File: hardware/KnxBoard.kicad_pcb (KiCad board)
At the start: 4 copper layers, 41.8 x 41.9 mm, 47 parts, among them IC0 STM32G491KEU6, IC1 NCN5130, J1 Conn_01x16, J2 Conn_01x16, J4 Conn_01x02_Male, X1 FA-238

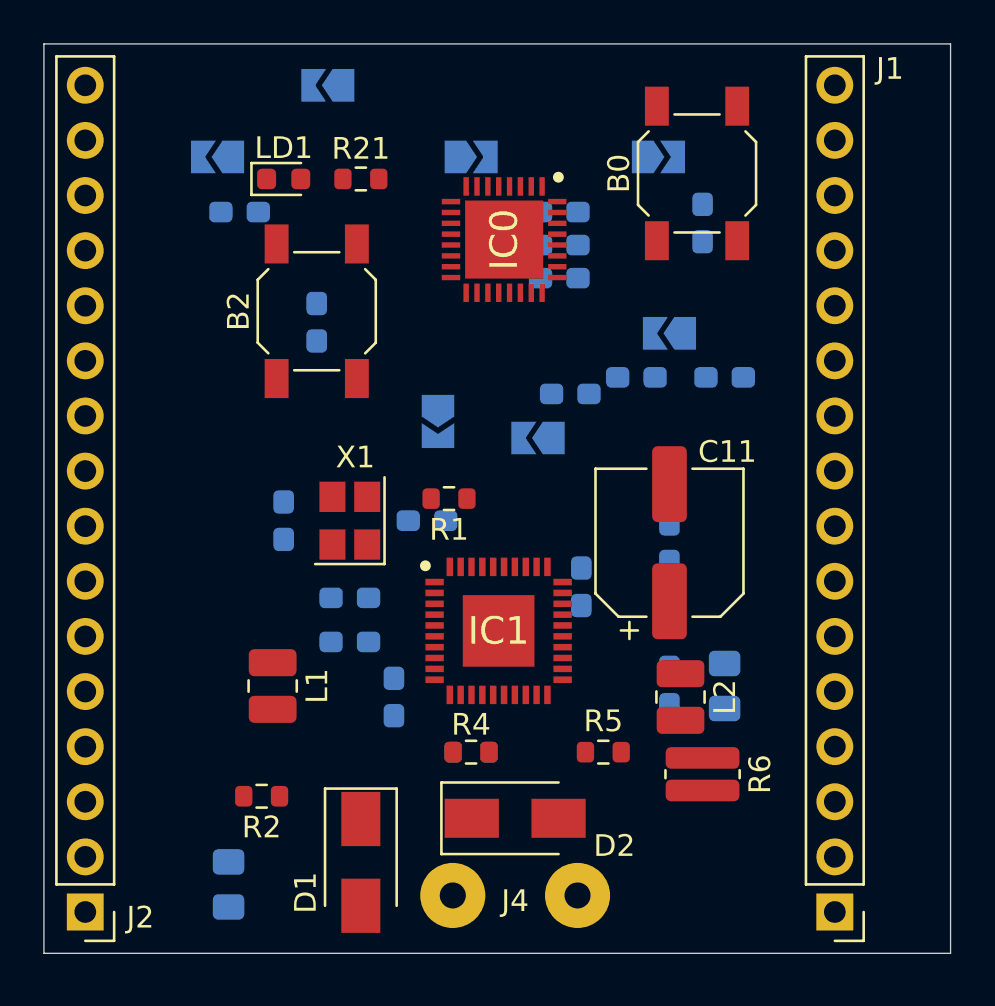
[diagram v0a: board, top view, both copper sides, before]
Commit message: Routage OK need check and mass and texts
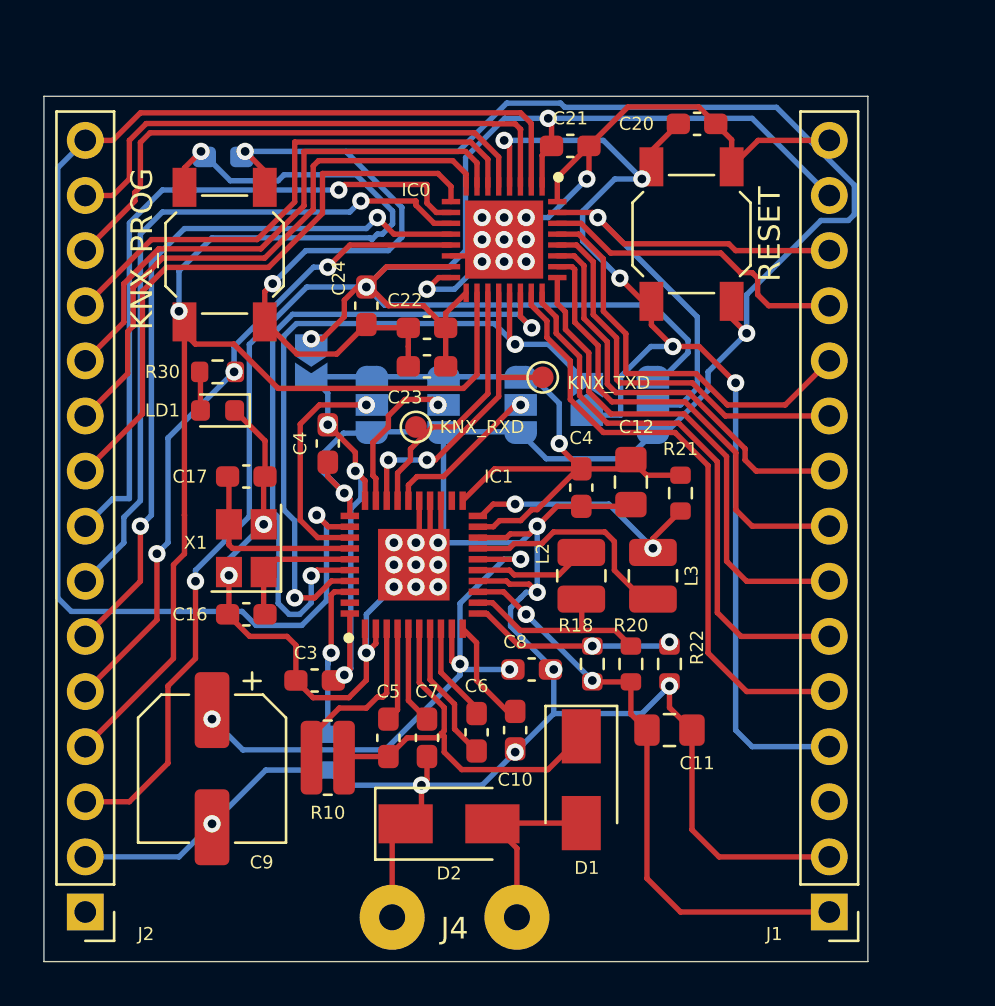
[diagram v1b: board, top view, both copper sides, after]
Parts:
- removed C1 (x2): 100 nF, Capacitor_SMD:C_0603_1608Metric_Pad1.08x0.95mm_HandSolder
- removed the C11 at (113.3, 55.4)
- removed C5_9: 100nF, Capacitor_SMD:C_0603_1608Metric_Pad1.08x0.95mm_HandSolder
- removed JP0, JP5: Bootloader, Jumper:SolderJumper-2_P1.3mm_Open_TrianglePad1.0x1.5mm
- added C20: 100 nF, Capacitor_SMD:C_0603_1608Metric_Pad1.08x0.95mm_HandSolder, F.Cu at (114.6, 36.1)
- added C8: 100nF 50V, Capacitor_SMD:C_0603_1608Metric_Pad1.08x0.95mm_HandSolder, F.Cu at (106.9, 61.2)
- added C9: 100uF 35V, Capacitor_SMD:CP_Elec_6.3x7.7, F.Cu at (92.2, 65.8)
- added JP3: Speed, Jumper:SolderJumper-3_P1.3mm_Open_RoundedPad1.0x1.5mm, B.Cu at (106.4, 49.0)
- added TP1: KNX_RXD, TestPoint:TestPoint_Pad_D1.0mm, F.Cu at (101.6, 50.0)
- added TP2: KNX_TXD, TestPoint:TestPoint_Pad_D1.0mm, F.Cu at (107.4, 47.8)
- C10: renamed from C12; value 1uF 35V ESR < 2ohm -> 1uF 50V ESR < 2ohm; moved to F.Cu
- C11: renamed from C19; moved to F.Cu
- C12: renamed from C20; moved to F.Cu
- C16, C17, C4: moved to F.Cu
- C21: renamed from C5; moved to F.Cu
- C22: renamed from C3; moved to F.Cu
- C23: renamed from C2; moved to F.Cu
- C24: renamed from C4; moved to F.Cu
- C3: renamed from C15; moved to F.Cu
- C4: renamed from C6; moved to F.Cu
- C5: renamed from C14; moved to F.Cu
- C6: renamed from C13; moved to F.Cu
- C7: renamed from C10; moved to F.Cu
- D1: value SS16 -> SS16T3G
- J1, J2: value Conn_01x16 -> Conn_01x15; footprint Connector_PinHeader_2.54mm:PinHeader_1x16_P2.54mm_Vertical -> Connector_PinHeader_2.54mm:PinHeader_1x15_P2.54mm_Vertical
- J4: value Conn_01x02_Male -> Conn_01x02
- JP1: value Bootflash -> Clock_8_16; footprint Jumper:SolderJumper-2_P1.3mm_Open_TrianglePad1.0x1.5mm -> Jumper:SolderJumper-3_P1.3mm_Open_RoundedPad1.0x1.5mm
- JP2: value RESETB_NRST -> Parity; footprint Jumper:SolderJumper-2_P1.3mm_Open_TrianglePad1.0x1.5mm -> Jumper:SolderJumper-3_P1.3mm_Open_RoundedPad1.0x1.5mm
- JP4: value Bootflash -> BootMode; footprint Jumper:SolderJumper-2_P1.3mm_Open_TrianglePad1.0x1.5mm -> Jumper:SolderJumper-3_P1.3mm_Open_RoundedPad1.0x1.5mm
- R22: renamed from R3; moved to F.Cu
- R3: renamed from R1; moved to B.Cu
- moved C11 21.5 mm to (113.3, 64.0), turned to 0 degrees
- moved JP4 21.0 mm to (112.5, 49.0), turned to 90 degrees
- moved R10 17.3 mm to (97.5, 65.3), turned to 0 degrees
- moved R18 16.4 mm to (109.7, 61.0), turned to -90 degrees
- moved C3 16.4 mm to (96.9, 61.7), turned to 0 degrees
- moved JP2 15.5 mm to (102.9, 49.0), turned to 90 degrees
- moved L2 15.1 mm to (109.2, 56.9)
- moved C4 14.1 mm to (97.5, 50.8), turned to -90 degrees
- moved R3 13.0 mm to (97.5, 65.0), turned to -90 degrees
- moved R21 12.5 mm to (113.8, 53.1), turned to 90 degrees
- moved JP1 12.3 mm to (99.6, 49.0), turned to 90 degrees
- moved C10 11.2 mm to (106.2, 64.0), turned to -90 degrees
- moved LD1 11.1 mm to (92.5, 49.3), turned to 180 degrees
- moved R30 11.1 mm to (92.5, 47.5)
- moved D1 10.9 mm to (109.2, 66.3)
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- renumbered C18 to C30, JP3 to JP7, L1 to L2, L2 to L3, R6 to R10, R2 to R18, R4 to R20, R5 to R21, R21 to R30
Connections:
- C10 pad 1: /KNXIFACE/Vfilt -> Net-(C10-Pad1)
- C4 pad 1: VDD -> +3V3
- D2 pad 1: /KNXIFACE/KNX+ -> GNDREF
- D2 pad 2: GNDREF -> /KNXIFACE/KNX+
- IC0 pad 19: KNX_RXD -> /KNXIFACE/KNX_RXD
- IC0 pad 20: KNX_TXD -> /KNXIFACE/KNX_TXD
- IC1 pad 10: /KNXIFACE/Vfilt -> Net-(C10-Pad1)
- IC1 pad 26: GNDREF -> Net-(IC1-Pad26)
- IC1 pad 27: KNX_RXD -> /KNXIFACE/KNX_RXD
- IC1 pad 28: KNX_TXD -> /KNXIFACE/KNX_TXD
- IC1 pad 29: GNDREF -> Net-(IC1-Pad29)
- IC1 pad 33: GNDREF -> Net-(JP1-Pad2)
- J1 pad 1: Prog -> +12V
- J1 pad 10: /MCU/PB4 -> /MCU/PB5
- J1 pad 11: /MCU/PB5 -> /MCU/PB6
- J1 pad 12: /MCU/PB6 -> /MCU/PB7
- J1 pad 13: /MCU/PB7 -> /MCU/PB8
- J1 pad 14: /MCU/PB8 -> VDD
- J1 pad 15: VDD -> GNDREF
- J1 pad 2: KNX_TXD -> GNDREF
- J1 pad 3: KNX_RXD -> unconnected-(J1-Pad3)
- J1 pad 4: KNX_RESETB -> NRST
- J1 pad 5: KNX_SAVEB -> /MCU/DEBUG_JTMS-SWDIO
- J1 pad 6: /MCU/DEBUG_JTMS-SWDIO -> /MCU/DEBUG_JTCK-SWCLK
- J1 pad 7: /MCU/DEBUG_JTCK-SWCLK -> /MCU/DEBUG_JTDI
- J1 pad 8: /MCU/DEBUG_JTDI -> /MCU/DEBUG_JTDA-SWO
- J1 pad 9: /MCU/DEBUG_JTDA-SWO -> /MCU/PB4
- J2 pad 1: +12V -> unconnected-(J2-Pad1)
- J2 pad 14: NRST -> /MCU/PF1
- J2 pad 15: /MCU/PF1 -> CLK16
- J2 pad 4: GNDREF -> Prog
- J4 pad 1: /KNXIFACE/KNX+ -> GNDREF
- J4 pad 2: GNDREF -> /KNXIFACE/KNX+
- JP1 pad 2: Net-(JP0-Pad1) -> Net-(JP1-Pad2)
- JP2 pad 1: NRST -> GNDREF
- JP2 pad 2: KNX_RESETB -> Net-(IC1-Pad29)
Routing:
- net GNDREF: track 0.00 -> 264.3 mm, vias 0 -> 34
- net VDD: track 0.00 -> 98.8 mm, vias 0 -> 4
- net Prog: track 0.00 -> 66.0 mm, vias 0 -> 2
- net CLK16: track 0.00 -> 65.1 mm, vias 0 -> 1
- net NRST: track 0.00 -> 53.9 mm, vias 0 -> 5
- net +3V3: track 0.00 -> 51.8 mm, vias 0 -> 4
- net /MCU/PA7: track 0.00 -> 33.5 mm, vias 0 -> 2
- net KNX_RESETB: track 0.00 -> 33.0 mm, vias 0 -> 2
- net /MCU/PA6: track 0.00 -> 32.5 mm, vias 0 -> 1
- net KNX_SAVEB: track 0.00 -> 32.0 mm, vias 0 -> 2
- net /MCU/PA5: track 0.00 -> 31.9 mm, vias 0 -> 1
- net Led: track 0.00 -> 30.7 mm, vias 0 -> 3
- net /MCU/DEBUG_JTMS-SWDIO: track 0.00 -> 28.2 mm
- net /MCU/PA4: track 0.00 -> 27.9 mm
- net +12V: track 0.00 -> 27.4 mm, vias 0 -> 2
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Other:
- board size 41.8 x 41.9 mm -> 38 x 39.9 mm
